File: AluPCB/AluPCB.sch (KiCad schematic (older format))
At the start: 83 parts, among them J1 CON_U, J2 CON_U, J3 CON_U, J4 GND, J5 VIN, Q1 AON6276, Q2 AON6276, Q3 AON6276, Q4 AON6276, Q5 AON6276, Q6 AON6276

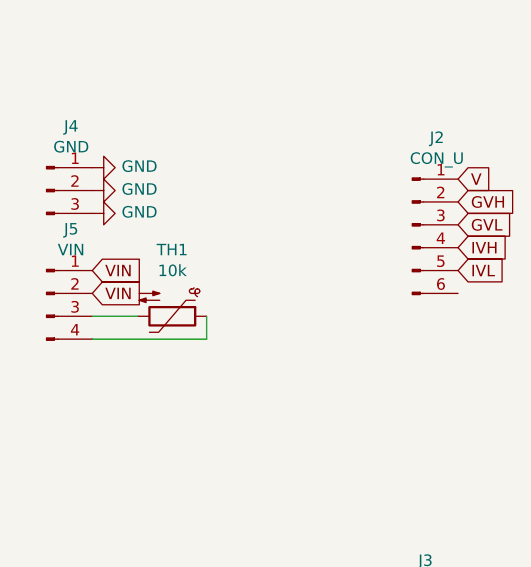
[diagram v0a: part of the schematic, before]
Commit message: wip
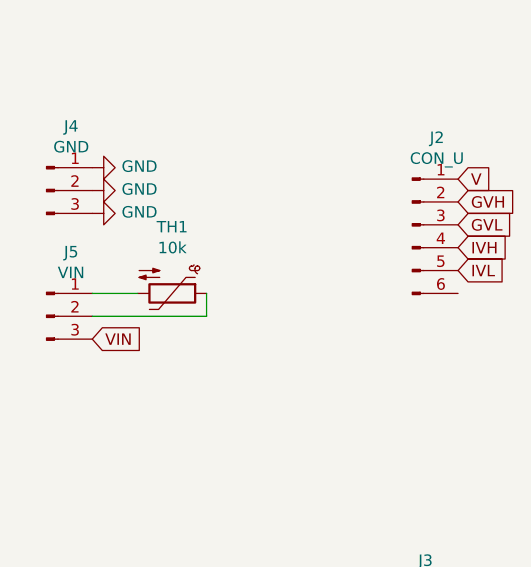
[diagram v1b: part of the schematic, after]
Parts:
- removed J5: VIN, Connector_PinSocket_2.00mm:PinSocket_1x04_P2.00mm_Vertical_SMD_Pin1Left, symbol Connector:Conn_01x04_Male
- added J5: VIN, Connector_PinSocket_2.00mm:PinSocket_1x03_P2.00mm_Vertical_SMD_Pin1Left, symbol Connector:Conn_01x03_Male
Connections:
- net VIN: now also J5.3 (Pin_3)
- net at TH1.1: now also J5.2 (Pin_2)
- net at TH1.2: now also J5.1 (Pin_1)
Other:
- moved on the sheet: TH1
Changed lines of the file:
@@
 L Device:Thermistor_NTC TH1
 U 1 1 5CDFE2AF
-P 1300 3750
-F 0 "TH1" V 1010 3750 50  0000 C CNN
-F 1 "10k" V 1101 3750 50  0000 C CNN
-F 2 "Resistor_SMD:R_0603_1608Metric" H 1300 3800 50  0001 C CNN
-F 3 "~" H 1300 3800 50  0001 C CNN
-	1    1300 3750
+P 1300 3650
+F 0 "TH1" V 1010 3650 50  0000 C CNN
+F 1 "10k" V 1101 3650 50  0000 C CNN
+F 2 "Resistor_SMD:R_0603_1608Metric" H 1300 3700 50  0001 C CNN
+F 3 "~" H 1300 3700 50  0001 C CNN
+	1    1300 3650
 	0    1    1    0
 $EndComp
 Wire Wire Line
-	1150 3750 950  3750
+	1150 3650 950  3650
 Wire Wire Line
-	1450 3750 1450 3850
+	1450 3650 1450 3750
 Wire Wire Line
-	1450 3850 950  3850
+	1450 3750 950  3750
 $Comp
 L power:GND #PWR0166
@@
 	0    -1   -1   0
 $EndComp
-Text GLabel 950  3550 2    50   Input ~ 0
-VIN
-Text GLabel 950  3650 2    50   Input ~ 0
+Text GLabel 950  3850 2    50   Input ~ 0
 VIN
 $Comp
@@
 $EndComp
 $Comp
-L Connector:Conn_01x04_Male J5
-U 1 1 5CE7B946
-P 750 3650
-F 0 "J5" H 858 3931 50  0000 C CNN
-F 1 "VIN" H 858 3840 50  0000 C CNN
-F 2 "Connector_PinSocket_2.00mm:PinSocket_1x04_P2.00mm_Vertical_SMD_Pin1Left" H 750 3650 50  0001 C CNN
-F 3 "~" H 750 3650 50  0001 C CNN
-	1    750  3650
-	1    0    0    -1
-$EndComp
-$Comp
 L power:GND #PWR0168
 U 1 1 5CE7D54B
@@
 	0    -1   -1   0
 $EndComp
+$Comp
+L Connector:Conn_01x03_Male J5
+U 1 1 5CCA217B
+P 750 3750
+F 0 "J5" H 858 4031 50  0000 C CNN
+F 1 "VIN" H 858 3940 50  0000 C CNN
+F 2 "Connector_PinSocket_2.00mm:PinSocket_1x03_P2.00mm_Vertical_SMD_Pin1Left" H 750 3750 50  0001 C CNN
+F 3 "~" H 750 3750 50  0001 C CNN
+	1    750  3750
+	1    0    0    -1
+$EndComp
 $EndSCHEMATC
